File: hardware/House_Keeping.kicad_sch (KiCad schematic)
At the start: 4 parts, among them Q7 SI2302DDS-T1-GE3, U15 CD4051BPWR, U16 CD4051BPWR

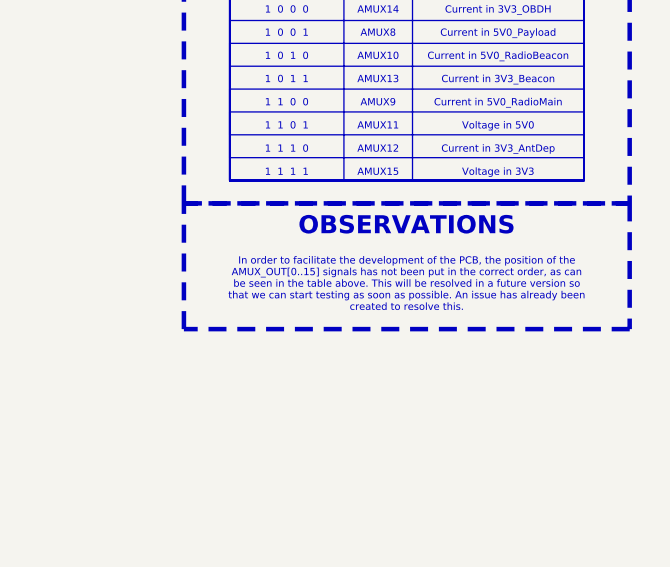
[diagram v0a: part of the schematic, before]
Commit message: hardware: Minor modifications for the upcoming release
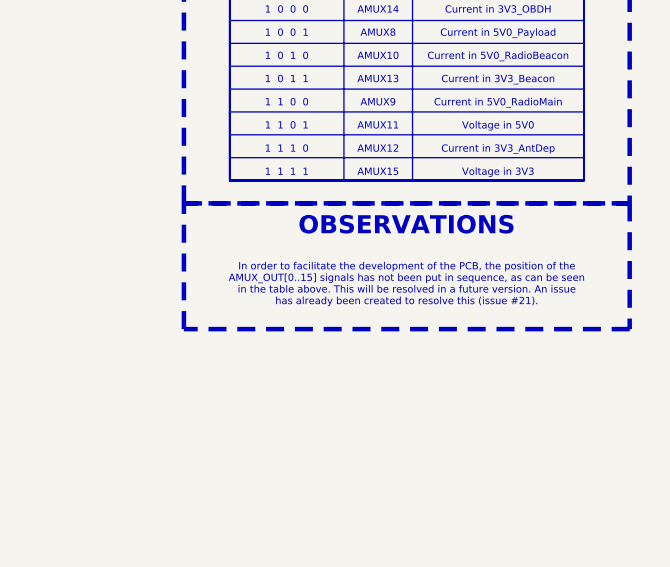
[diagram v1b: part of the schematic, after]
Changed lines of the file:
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@@
     (effects (font (size 0.8 0.8) (color 0 0 0 1)))
   )
-  (text_box "In order to facilitate the development of the PCB, the position of the AMUX_OUT[0..15] signals has not been put in the correct order, as can be seen in the table above. This will be resolved in a future version so that we can start testing as soon as possible. An issue has already been created to resolve this."
+  (text_box "In order to facilitate the development of the PCB, the position of the AMUX_OUT[0..15] signals has not been put in sequence, as can be seen in the table above. This will be resolved in a future version. An issue has already been created to resolve this (issue #21)."
     (at 236.22 68.58 0) (size 46.99 10.16)
     (stroke (width -0.0001) (type default))
